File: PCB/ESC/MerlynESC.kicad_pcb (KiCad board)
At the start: 4 copper layers, 30.5 x 31.9 mm, 155 parts, among them M1 BLDC Motor, M2 BLDC Motor, M3 BLDC Motor, M4 BLDC Motor, Q1 JMSL0302AU, Q10 JMSL0302AU, Q11 JMSL0302AU, Q12 JMSL0302AU, Q13 JMSL0302AU, Q14 JMSL0302AU, Q15 JMSL0302AU, Q16 JMSL0302AU, Q17 JMSL0302AU, Q18 JMSL0302AU, Q19 JMSL0302AU, Q2 JMSL0302AU, Q20 JMSL0302AU, Q21 JMSL0302AU, Q22 JMSL0302AU, Q23 JMSL0302AU, Q24 JMSL0302AU, Q3 JMSL0302AU, Q4 JMSL0302AU, Q5 JMSL0302AU, Q6 JMSL0302AU, Q7 JMSL0302AU, Q8 JMSL0302AU, Q9 JMSL0302AU, U1 HT75C0-1, U10 EG6288, U11 EFM8BB21F16G, U2 HT7533-1, U3 EFM8BB21F16G, U4 EG6288, U5 EG6288, U6 EFM8BB21F16G, U7 INA139NA, U8 EG6288, U9 EFM8BB21F16G

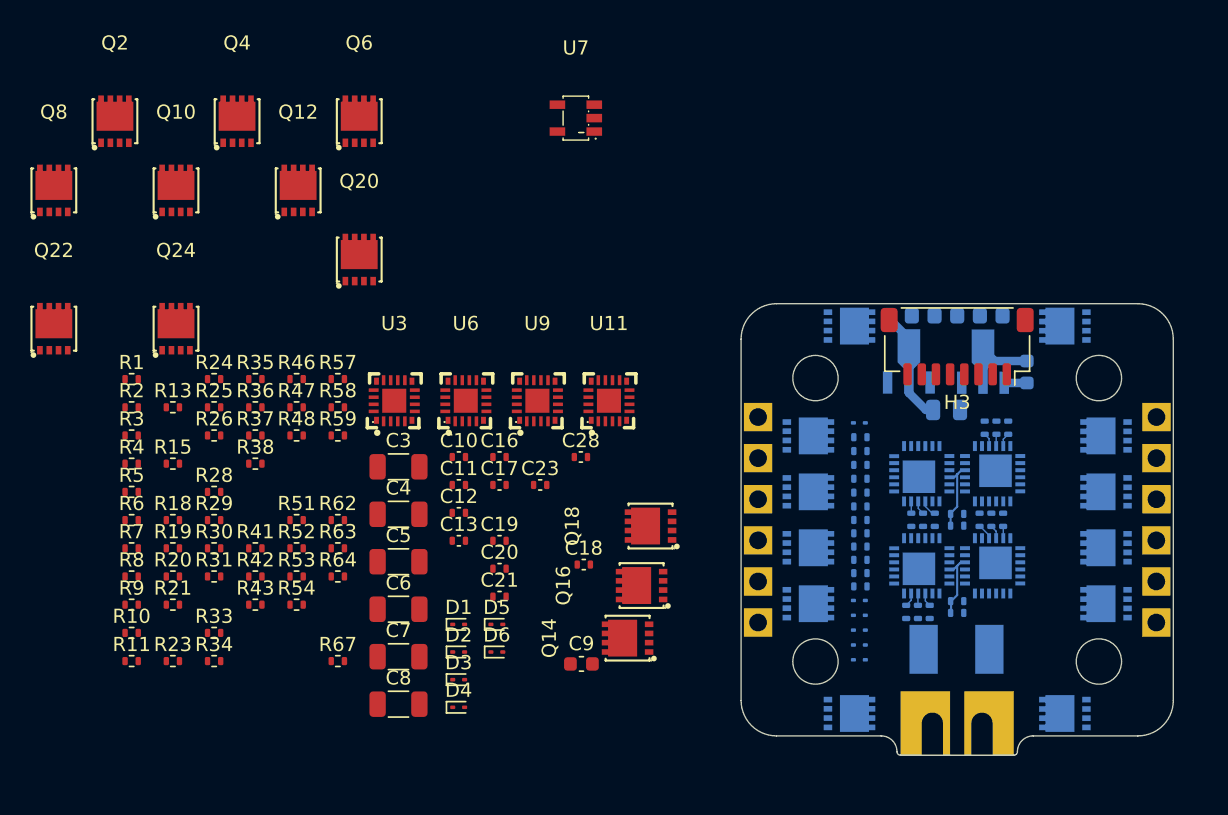
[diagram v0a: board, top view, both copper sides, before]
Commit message: checkpoint
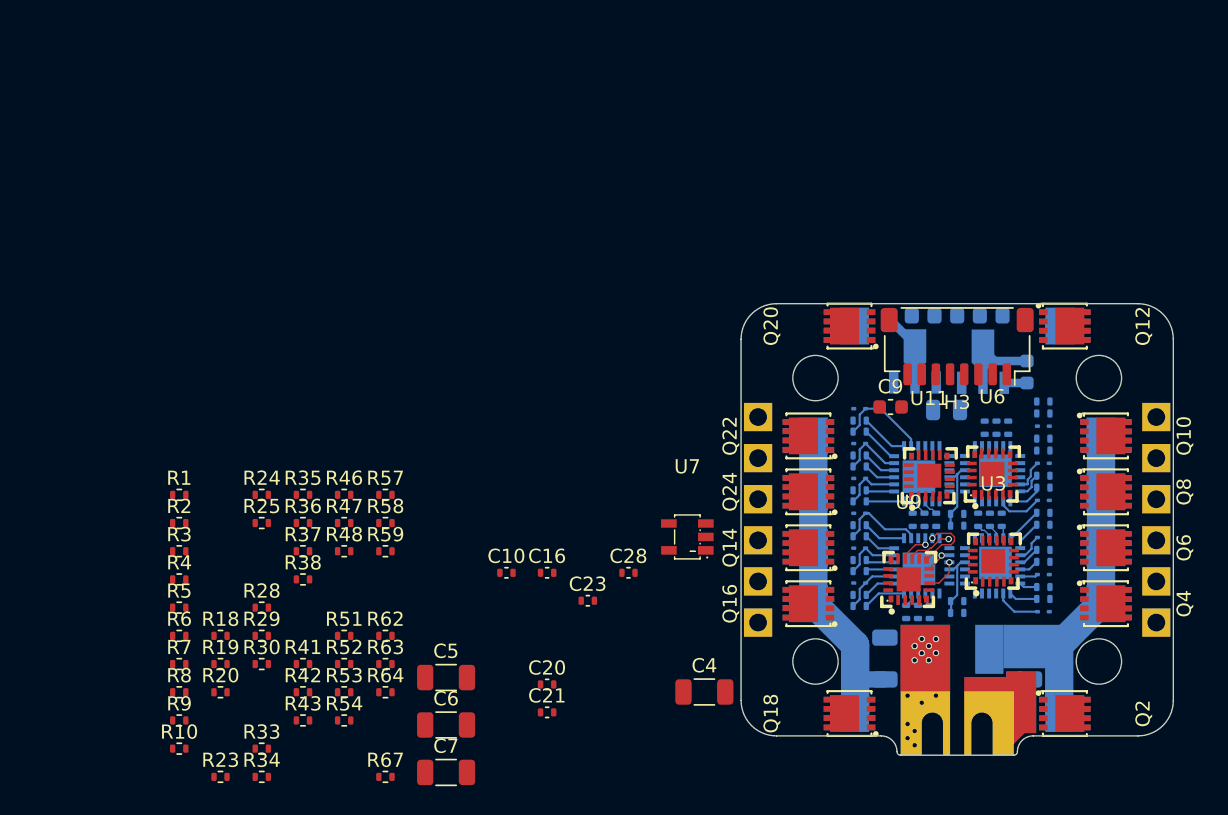
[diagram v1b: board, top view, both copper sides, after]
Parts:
- C11, C12, C13, C17, C18, C19, C3, C8, D1, D2, D3, D4, D5, D6, R11, R13, R15, R21, R26, R31: moved to B.Cu
- moved Q2 79.0 mm to (163.0, 115.6), turned to -90 degrees
- moved Q8 77.2 mm to (165.9, 100.0), turned to -90 degrees
- moved Q4 70.1 mm to (165.9, 107.9), turned to -90 degrees
- moved Q10 67.9 mm to (165.9, 96.0), turned to -90 degrees
- moved R11 64.5 mm to (161.5, 107.5), turned to 180 degrees
- moved R13 62.4 mm to (161.5, 104.9), turned to 180 degrees
- moved R21 62.0 mm to (161.5, 99.7), turned to 180 degrees
- moved R15 61.6 mm to (161.5, 102.3), turned to 180 degrees
- moved Q6 60.7 mm to (165.9, 103.9), turned to -90 degrees
- moved R31 59.6 mm to (161.5, 94.4), turned to 180 degrees
- moved R26 58.5 mm to (161.5, 97.1), turned to 180 degrees
- moved Q12 54.9 mm to (163.0, 88.3), turned to -90 degrees
- moved Q22 53.8 mm to (144.9, 96.0), turned to 90 degrees
- moved Q24 46.1 mm to (144.9, 100.0), turned to 90 degrees
- moved C8 44.6 mm to (160.5, 111.7), turned to 90 degrees
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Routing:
- net +BATT: track 5.97 -> 49.5 mm
- net Net-(D10-K): track 0.00 -> 6.58 mm
- net Net-(D7-K): track 0.00 -> 6.08 mm
- net M3_HIN2: track 0.00 -> 4.63 mm, vias 0 -> 1
- net Net-(D11-K): track 0.00 -> 4.57 mm
- net GND: track 1.61 -> 6.06 mm
- net Net-(D8-K): track 0.00 -> 4.20 mm
- net Net-(D9-K): track 0.00 -> 4.19 mm
- net Net-(D12-K): track 0.00 -> 4.17 mm
- net M4_H01: track 0.00 -> 3.41 mm
- net M3_LIN1: track 0.00 -> 3.28 mm, vias 0 -> 1
- net Net-(D1-K): track 0.00 -> 3.23 mm
- net Net-(D4-K): track 0.00 -> 3.18 mm
- net M3_H01: track 0.00 -> 3.05 mm
- net Net-(U8-VS3): track 0.00 -> 3.03 mm
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
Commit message: checkpoint
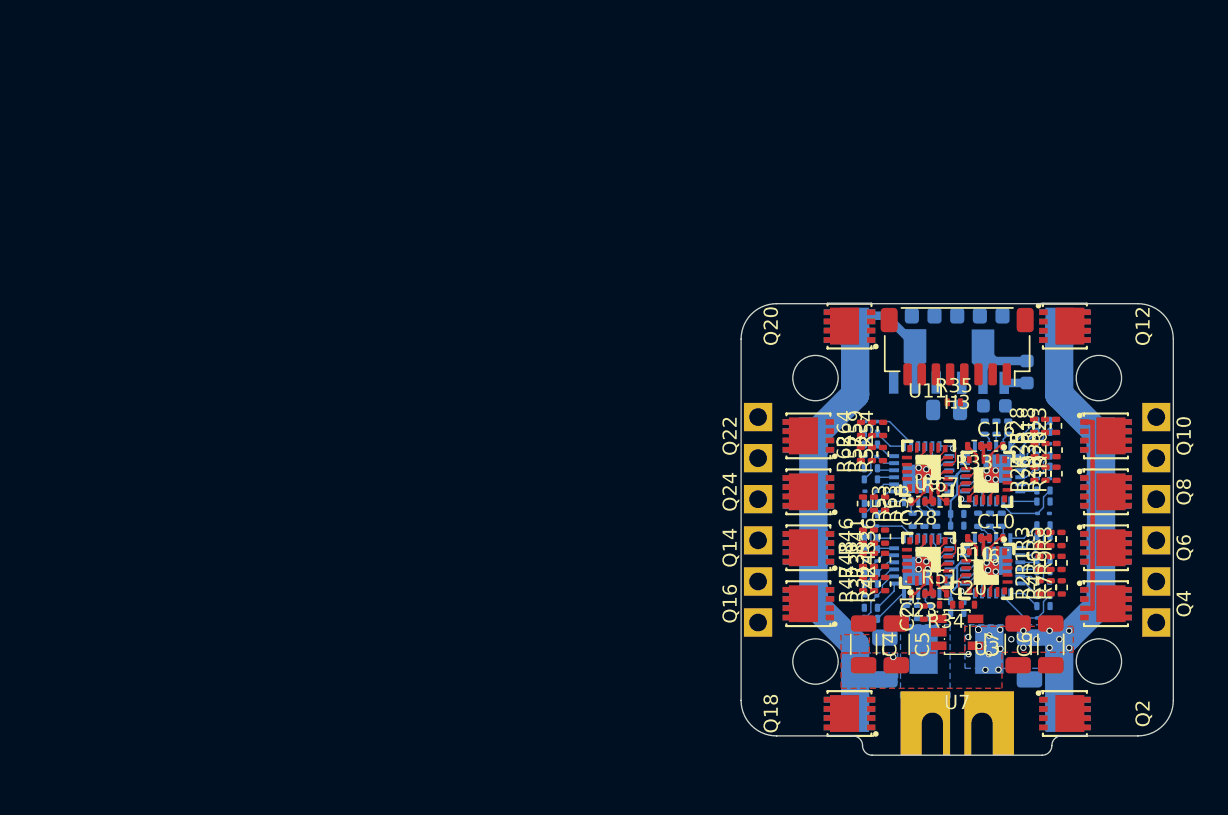
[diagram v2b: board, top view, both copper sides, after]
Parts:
- C9: moved to B.Cu
- moved R23 64.0 mm to (162.4, 95.3), turned to 90 degrees
- moved R9 63.3 mm to (162.8, 105.0), turned to 90 degrees
- moved R8 63.2 mm to (162.8, 103.3), turned to 90 degrees
- moved R7 62.5 mm to (162.8, 106.7), turned to 90 degrees
- moved R6 61.7 mm to (162.0, 105.0), turned to 90 degrees
- moved R5 61.7 mm to (162.0, 103.3), turned to 90 degrees
- moved R4 61.5 mm to (162.0, 106.7), turned to 90 degrees
- moved R20 61.4 mm to (162.4, 97.0), turned to 90 degrees
- moved R1 60.9 mm to (161.2, 105.0), turned to 90 degrees
- moved R2 60.9 mm to (161.2, 106.7), turned to 90 degrees
- moved R3 60.7 mm to (161.2, 103.3), turned to 90 degrees
- moved R19 60.5 mm to (162.4, 98.7), turned to 90 degrees
- moved R18 60.0 mm to (161.6, 95.3), turned to 90 degrees
- moved R10 58.0 mm to (156.6, 103.2), turned to 180 degrees
- moved R30 57.3 mm to (161.7, 97.0), turned to 90 degrees
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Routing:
- net +BATT: track 49.5 -> 71.2 mm, vias 0 -> 22
- net GND: track 6.06 -> 27.8 mm, vias 0 -> 16
- net +3.3V: track 0.00 -> 6.34 mm
- net Net-(D6-K): track 0.00 -> 4.03 mm
- net M4_HIN3: track 0.00 -> 2.85 mm, vias 0 -> 1
- net M1_LIN1: track 0.00 -> 2.81 mm, vias 0 -> 1
- net M2_LIN1: track 0.00 -> 2.81 mm, vias 0 -> 1
- net M4_LIN1: track 0.00 -> 2.81 mm, vias 0 -> 1
- net M3_HIN2: track 4.63 -> 1.87 mm
- net M2_HIN3: track 0.00 -> 2.63 mm, vias 0 -> 1
- net Net-(U5-VS3): track 0.00 -> 2.62 mm
- net M1_HIN3: track 0.00 -> 2.61 mm, vias 0 -> 1
- net M3_HIN3: track 0.00 -> 2.60 mm, vias 0 -> 1
- net M4_LIN2: track 0.00 -> 2.32 mm, vias 0 -> 1
- net M2_LIN2: track 0.00 -> 2.32 mm, vias 0 -> 1
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- added copper zone on B.Cu, net +BATT
- added copper zone on F.Cu, net +BATT
- added copper zone on B.Cu, net Net-(BT1-+)
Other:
- outline, holes or cut-outs redrawn
